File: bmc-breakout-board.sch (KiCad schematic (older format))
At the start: 49 parts, among them J1 PinHeader_2x4, J10 PinHeader_2x4, J11 PinHeader_2x05, J12 61300411121, J13 0473460001, J14 PCIE_BUS_x1, J15 0473460001, J16 PinHeader_1x07, J17 UE27AC54100, J2 PinHeader_2x13, J3 PinHeader_2x08, J4 61300411121, J5 ME1016813401101, J6 61300411121, J7 DC_SOCKET, J8 PinHeader_2x05, J9 PinHeader_1x07, Q1 SI2337DS, U1 FT234XD-R

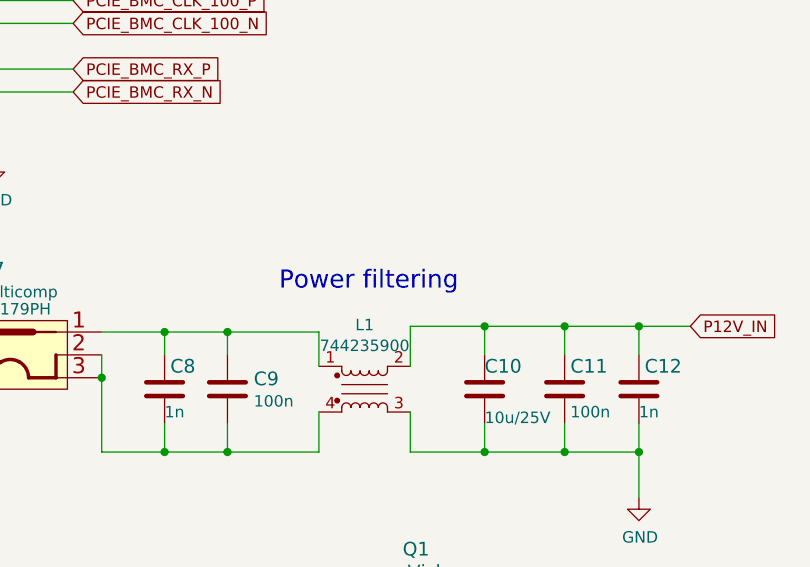
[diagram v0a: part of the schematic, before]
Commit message: Update component arrangement
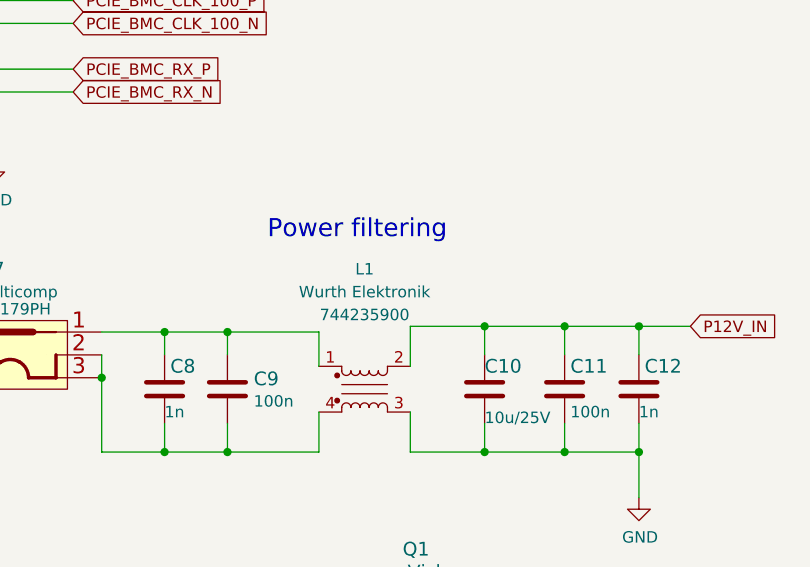
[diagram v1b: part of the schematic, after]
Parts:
- removed L1: 744235900, bmc-breakout-board-footprints:744235900, symbol bmc-breakout-board:744235900
- added L1: 744235900, antmicro-footprints:744235900, symbol antmicroFixedInductors:744235900
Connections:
- net GND: now also L1.3
- net P12V_IN: now also L1.2
- net at C8.1, C9.1, J7.1: now also L1.1
- net at C8.2, C9.2, J7.2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: now also L1.4
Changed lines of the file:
@@
-$EndComp
-$Comp
-L bmc-breakout-board:744235900 L1
-U 1 1 621486C2
-P 13925 4450
-F 0 "L1" H 13925 4731 50  0000 C CNN
-F 1 "744235900" H 13925 4640 50  0000 C CNN
-F 2 "bmc-breakout-board-footprints:744235900" H 13925 4450 50  0001 C CNN
-F 3 "~" H 13925 4450 50  0001 C CNN
-F 4 "Wurth Elektronik" H 13925 4450 50  0001 C CNN "Manufacturer"
-F 5 "744235900" H 13925 4450 50  0001 C CNN "MPN"
-	1    13925 4450
-	1    0    0    -1
 $EndComp
 $Comp
@@
 Text GLabel 6125 1575 2    50   Input ~ 0
 P12V_AUX
-Text Notes 13550 4025 0    79   ~ 0
+Text Notes 13500 3800 0    79   ~ 0
 Power filtering
 Connection ~ 13325 4725
@@
 Text Notes 11600 4350 0    79   ~ 0
 12VDC IN
+$Comp
+L antmicroFixedInductors:744235900 L1
+U 1 1 614300DC
+P 13925 4450
+F 0 "L1" H 13925 4975 50  0000 C CNN
+F 1 "744235900" H 13925 4275 50  0001 C CNN
+F 2 "antmicro-footprints:744235900" H 14525 4950 50  0001 C CNN
+F 3 "https://www.we-online.de/katalog/datasheet/744235900.pdf" H 13925 4450 50  0001 C CNN
+F 4 "Wurth Elektronik" H 13925 4875 50  0000 C CNN "Manufacturer"
+F 5 "744235900" H 13925 4775 50  0000 C CNN "MPN"
+F 6 "2A" H 14000 5100 50  0001 C CNN "MaxCur"
+F 7 "3.2x4.5" H 14075 5025 50  0001 C CNN "Size"
+F 8 "300n/2A" H 14150 4675 50  0001 C CNN "Val"
+	1    13925 4450
+	1    0    0    -1
+$EndComp
 $EndSCHEMATC
